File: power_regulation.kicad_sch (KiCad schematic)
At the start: 120 parts, among them IC3 NCV8184DR2G, IC4 MIE1W0505BGLVH-3R-P, J10 Conn_01x02_Pin, J7 V_bat_secondary, J8 Conn_01x02_Pin, J9 Conn_01x02_Pin, U10 OPA2387DR, U11 TPS7A2055PDBVR, U12 AP7361C-33Y5-13, U13 TPS7A2050PDBVR, U14 TPS7A2033PDBVR, U15 TPS7A2018PDBVRG4, U16 TLV75733PDYDR, U17 TPS7A2050PDBVR, U18 TPS7A2055PDBVR, U19 TPS7A2033PDBVR, U20 TPS7A2045PDBVR, U7 MCP1502T-50E/CHY, U8 TPS62933, U9 TPS62933

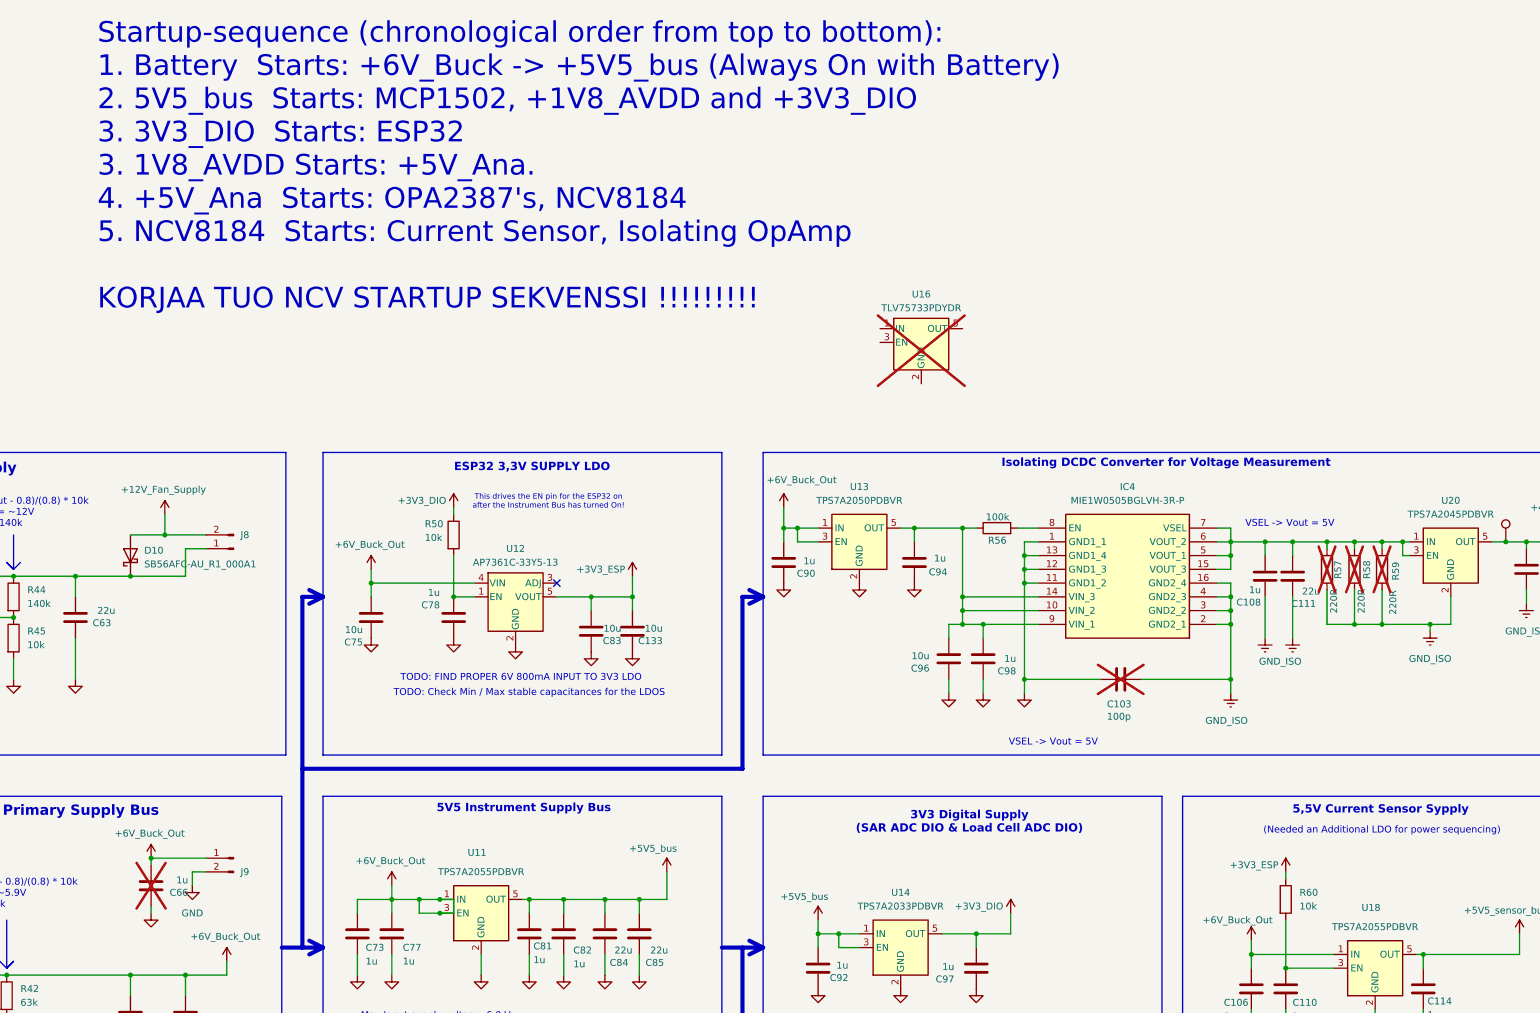
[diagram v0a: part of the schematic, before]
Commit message: Minor improvements
[KiCad Version: 10.0.3]
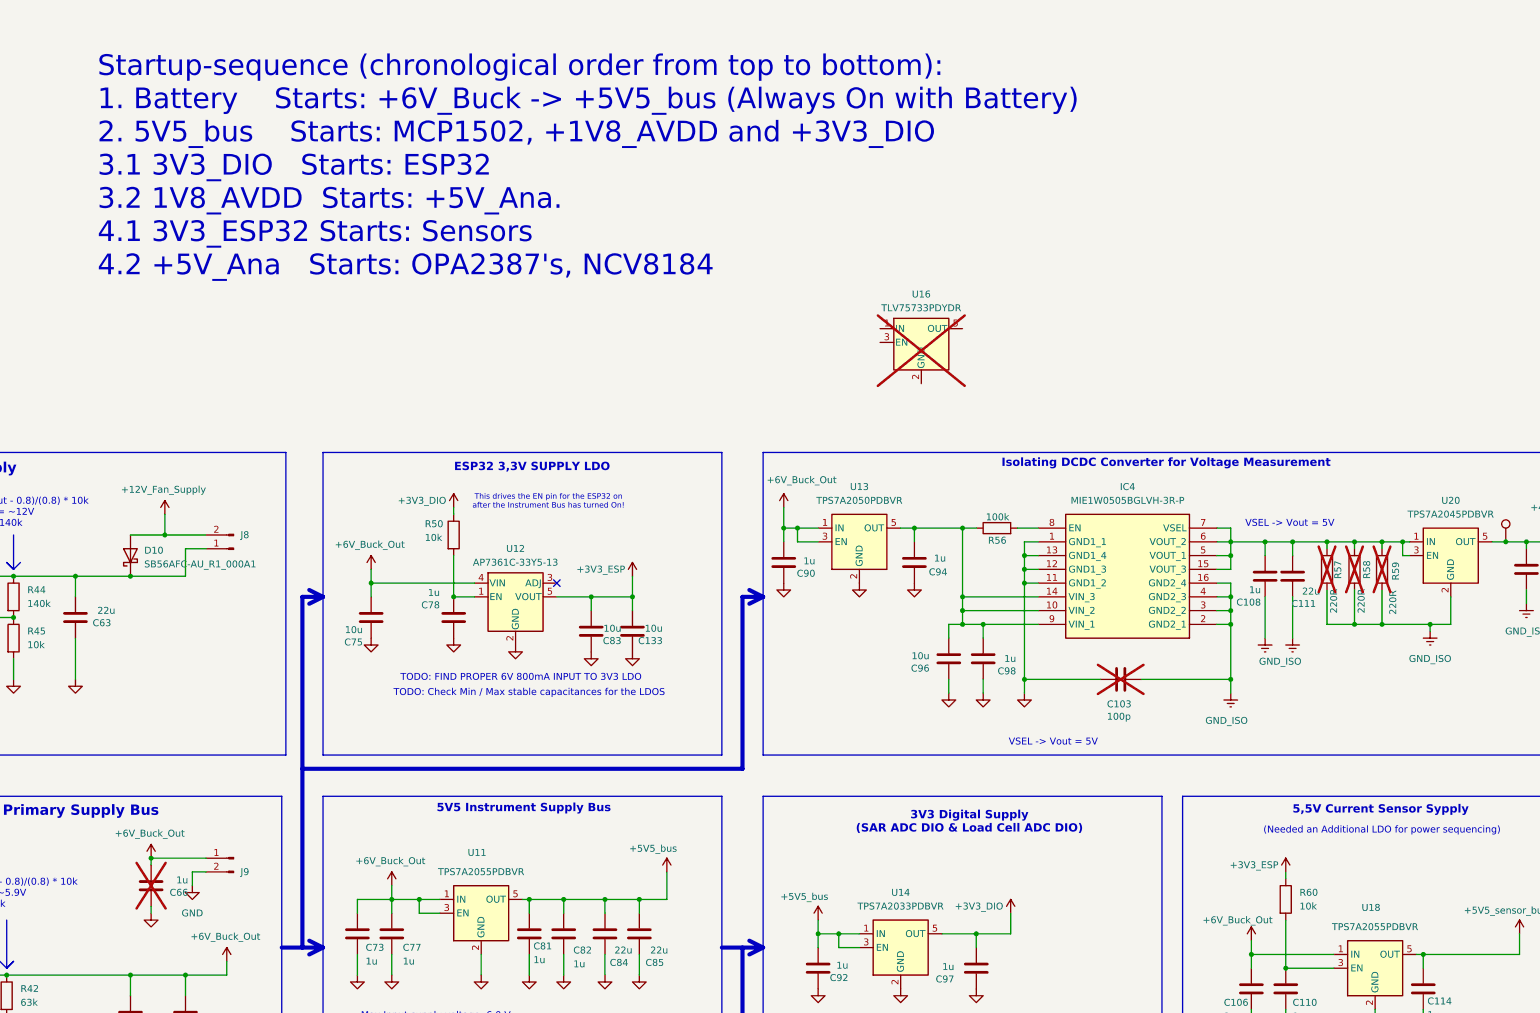
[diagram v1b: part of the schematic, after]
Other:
- note added: "Startup-sequence (chronological order from top to bottom): 1. Battery Starts: +6V_Buck -> +5V5_bus (Always On with Battery) 2. 5V5_bus Starts: MCP1502, +1V8_AVDD and +3V3_DIO 3.1 3V3_DIO Starts: ESP32 3.2 1V8_AVDD Starts: +5V_Ana. 4.1 3V3_ESP32 Starts: Sensors 4.2 +5V_Ana Starts: OPA2387's, NCV8184"
- note removed: "Startup-sequence (chronological order from top to bottom): 1. Battery Starts: +6V_Buck -> +5V5_bus (Always On with Battery) 2. 5V5_bus Starts: MCP1502, +1V8_AVDD and +3V3_DIO 3. 3V3_DIO Starts: ESP32 3. 1V8_AVDD Starts: +5V_Ana. 4. +5V_Ana Starts: OPA2387's, NCV8184 5. NCV8184 Starts: Current Sensor, Isolating OpAmp KORJAA TUO NCV STARTUP SEKVENSSI !!!!!!!!!"
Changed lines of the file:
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@@
 		)
 	)
-	(text "Startup-sequence (chronological order from top to bottom):\n1. Battery  Starts: +6V_Buck -> +5V5_bus (Always On with Battery) \n2. 5V5_bus  Starts: MCP1502, +1V8_AVDD and +3V3_DIO\n3. 3V3_DIO  Starts: ESP32\n3. 1V8_AVDD Starts: +5V_Ana.\n4. +5V_Ana  Starts: OPA2387's, NCV8184\n5. NCV8184  Starts: Current Sensor, Isolating OpAmp\n\nKORJAA TUO NCV STARTUP SEKVENSSI !!!!!!!!!"
+	(text "Startup-sequence (chronological order from top to bottom):\n1. Battery    Starts: +6V_Buck -> +5V5_bus (Always On with Battery) \n2. 5V5_bus    Starts: MCP1502, +1V8_AVDD and +3V3_DIO\n3.1 3V3_DIO   Starts: ESP32\n3.2 1V8_AVDD  Starts: +5V_Ana.\n4.1 3V3_ESP32 Starts: Sensors\n4.2 +5V_Ana   Starts: OPA2387's, NCV8184\n"
 		(exclude_from_sim no)
 		(at 124.714 -33.782 0)
@@
 	)
 	(junction
-		(at 187.96 101.6)
-		(diameter 0)
-		(color 0 0 0 0)
-	)
-	(junction
 		(at 162.56 161.29)
 		(diameter 0)
@@
 	)
 	(junction
-		(at 187.96 104.14)
-		(diameter 0)
-		(color 0 0 0 0)
-	)
-	(junction
 		(at 302.26 228.6)
 		(diameter 0)
@@
 	(wire
 		(pts
-			(xy 187.96 101.6) (xy 190.5 101.6)
-		)
-		(stroke
-			(width 0)
-			(type default)
-		)
-	)
-	(wire
-		(pts
 			(xy 62.23 57.15) (xy 62.23 59.69)
 		)
@@
 	(wire
 		(pts
-			(xy 190.5 101.6) (xy 190.5 104.14)
-		)
-		(stroke
-			(width 0)
-			(type default)
-		)
-	)
-	(wire
-		(pts
 			(xy 102.87 115.57) (xy 107.95 115.57)
 		)
@@
 		)
 		(stroke
-			(width 0)
-			(type default)
-		)
-	)
-	(wire
-		(pts
-			(xy 187.96 104.14) (xy 190.5 104.14)
-		)
-		(stroke
